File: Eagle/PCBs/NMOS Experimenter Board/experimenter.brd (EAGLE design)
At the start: 77.5 x 99.1 mm, 1441 parts, among them Q10 2N7002, Q11 2N7002, Q12 2N7002, Q13 2N7002, Q14 2N7002, Q15 2N7002, Q16 2N7002, Q17 2N7002, Q18 2N7002, Q19 2N7002, Q2 2N7002, Q20 2N7002, Q21 2N7002, Q22 2N7002, Q23 2N7002, Q24 2N7002, Q25 2N7002, Q26 2N7002, Q27 2N7002, Q28 2N7002, Q29 2N7002, Q3 2N7002, Q30 2N7002, Q31 2N7002, Q32 2N7002, Q33 2N7002, Q34 2N7002, Q35 2N7002, Q36 2N7002, Q37 2N7002, Q38 2N7002, Q39 2N7002, Q4 2N7002, Q40 2N7002, Q41 2N7002, Q42 2N7002, Q43 2N7002, Q44 2N7002, Q45 2N7002, Q46 2N7002, Q47 2N7002, Q48 2N7002, Q49 2N7002, Q5 2N7002, Q50 2N7002, Q51 2N7002, Q52 2N7002, Q53 2N7002, Q54 2N7002, Q55 2N7002, Q56 2N7002, Q57 2N7002, Q58 2N7002, Q59 2N7002, Q6 2N7002, Q60 2N7002, Q61 2N7002, Q62 2N7002, Q63 2N7002, Q64 2N7002, Q65 2N7002, Q66 2N7002, Q67 2N7002, Q68 2N7002, Q69 2N7002, Q7 2N7002, Q70 2N7002, Q71 2N7002, Q72 2N7002, Q73 2N7002, Q8 2N7002, Q9 2N7002, U1 74HC14PW, U2 74HC14PW

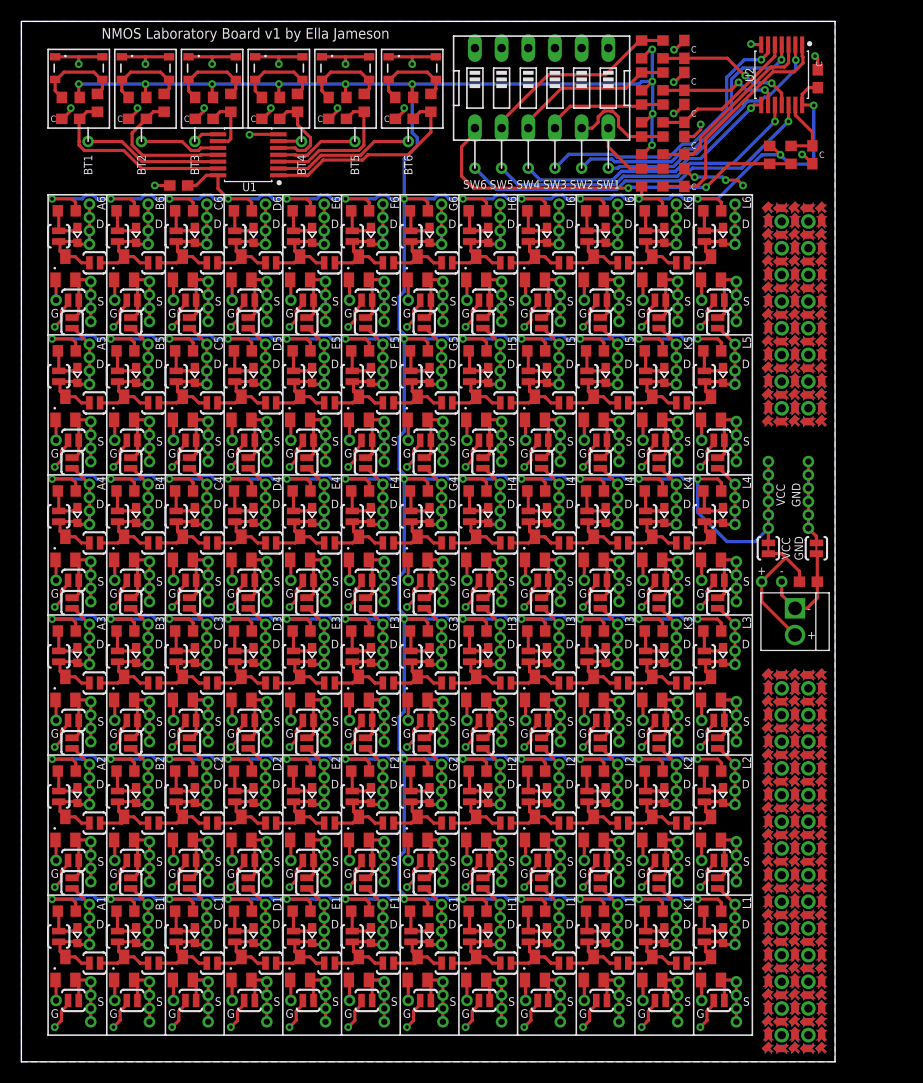
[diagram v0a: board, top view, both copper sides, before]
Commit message: Start rework on experimenter
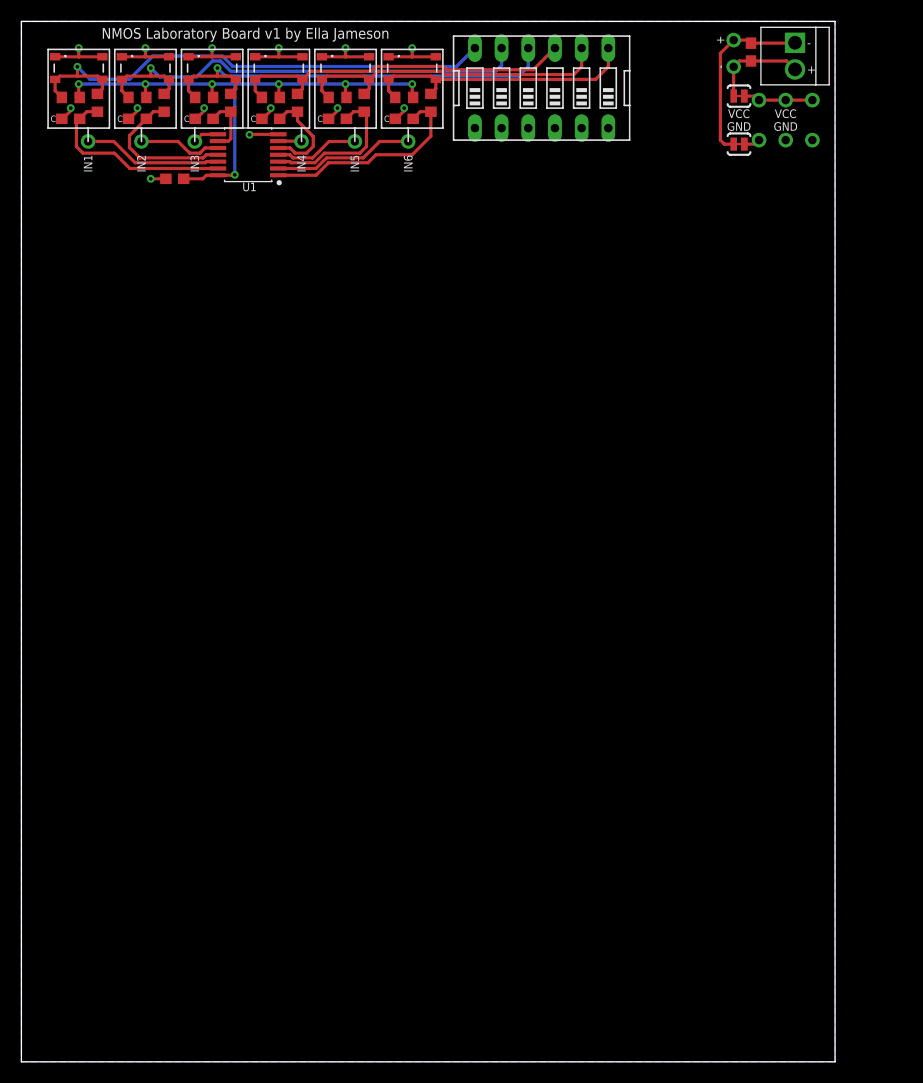
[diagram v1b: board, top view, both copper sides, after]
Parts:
- removed C10, C12, C13, C14, C15, C6, C8: 0.1u, ellajameson-core:C0603
- removed D10, D11, D12, D13, D14, D15, D16, D17, D18, D19, D2, D20, D21, D22, D23, D24, D25, D26, D27, D28, D29, D3, D30, D31, D32, D33, D34, D35, D36, D37, D38, D39, D4, D40, D41, D42, D43, D44, D45, D46, D47, D48, D49, D5, D50, D51, D52, D53, D54, D55, D56, D57, D58, D59, D6, D60, D61, D62, D63, D64, D65, D66, D67, D68, D69, D7, D70, D71, D72, D73, D8, D9: (no value), ellajameson-core:CHIP-LED0603
- removed DRAINA10, DRAINA11, DRAINA12, DRAINA13, DRAINA14, DRAINA15, DRAINA16, DRAINA17, DRAINA18, DRAINA19, DRAINA2, DRAINA20, DRAINA21, DRAINA22, DRAINA23, DRAINA24, DRAINA25, DRAINA26, DRAINA27, DRAINA28, DRAINA29, DRAINA3, DRAINA30, DRAINA31, DRAINA32, DRAINA33, DRAINA34, DRAINA35, DRAINA36, DRAINA37, DRAINA38, DRAINA39, DRAINA4, DRAINA40, DRAINA41, DRAINA42, DRAINA43, DRAINA44, DRAINA45, DRAINA46, DRAINA47, DRAINA48, DRAINA49, DRAINA5, DRAINA50, DRAINA51, DRAINA52, DRAINA53, DRAINA54, DRAINA55, DRAINA56, DRAINA57, DRAINA58, DRAINA59, DRAINA6, DRAINA60, DRAINA61, DRAINA62, DRAINA63, DRAINA64, DRAINA65, DRAINA66, DRAINA67, DRAINA68, DRAINA69, DRAINA7, DRAINA70, DRAINA71, DRAINA72, DRAINA73, DRAINA8, DRAINA9, DRAINB10, DRAINB11, DRAINB12, DRAINB13, DRAINB14, DRAINB15, DRAINB16, DRAINB17, DRAINB18, DRAINB19, DRAINB2, DRAINB20, DRAINB21, DRAINB22, DRAINB23, DRAINB24, DRAINB25, DRAINB26, DRAINB27, DRAINB28, DRAINB29, DRAINB3, DRAINB30, DRAINB31, DRAINB32, DRAINB33, DRAINB34, DRAINB35, DRAINB36, DRAINB37, DRAINB38, DRAINB39, DRAINB4, DRAINB40, DRAINB41, DRAINB42, DRAINB43, DRAINB44, DRAINB45, DRAINB46, DRAINB47, DRAINB48, DRAINB49, DRAINB5, DRAINB50, DRAINB51, DRAINB52, DRAINB53, DRAINB54, DRAINB55, DRAINB56, DRAINB57, DRAINB58, DRAINB59, DRAINB6, DRAINB60, DRAINB61, DRAINB62, DRAINB63, DRAINB64, DRAINB65, DRAINB66, DRAINB67, DRAINB68, DRAINB69, DRAINB7, DRAINB70, DRAINB71, DRAINB72, DRAINB73, DRAINB8, DRAINB9, DRAINC10, DRAINC11, DRAINC12, DRAINC13, DRAINC14, DRAINC15, DRAINC16, DRAINC17, DRAINC18, DRAINC19, DRAINC2, DRAINC20, DRAINC21, DRAINC22, DRAINC23, DRAINC24, DRAINC25, DRAINC26, DRAINC27, DRAINC28, DRAINC29, DRAINC3, DRAINC30, DRAINC31, DRAINC32, DRAINC33, DRAINC34, DRAINC35, DRAINC36, DRAINC37, DRAINC38, DRAINC39, DRAINC4, DRAINC40, DRAINC41, DRAINC42, DRAINC43, DRAINC44, DRAINC45, DRAINC46, DRAINC47, DRAINC48, DRAINC49, DRAINC5, DRAINC50, DRAINC51, DRAINC52, DRAINC53, DRAINC54, DRAINC55, DRAINC56, DRAINC57, DRAINC58, DRAINC59, DRAINC6, DRAINC60, DRAINC61, DRAINC62, DRAINC63, DRAINC64, DRAINC65, DRAINC66, DRAINC67, DRAINC68, DRAINC69, DRAINC7, DRAINC70, DRAINC71, DRAINC72, DRAINC73, DRAINC8, DRAINC9, DRAIND10, DRAIND11, DRAIND12, DRAIND13, DRAIND14, DRAIND15, DRAIND16, DRAIND17, DRAIND18, DRAIND19, DRAIND2, DRAIND20, DRAIND21, DRAIND22, DRAIND23, DRAIND24, DRAIND25, DRAIND26, DRAIND27, DRAIND28, DRAIND29, DRAIND3, DRAIND30, DRAIND31, DRAIND32, DRAIND33, DRAIND34, DRAIND35, DRAIND36, DRAIND37, DRAIND38, DRAIND39, DRAIND4, DRAIND40, DRAIND41, DRAIND42, DRAIND43, DRAIND44, DRAIND45, DRAIND46, DRAIND47, DRAIND48, DRAIND49, DRAIND5, DRAIND50, DRAIND51, DRAIND52, DRAIND53, DRAIND54, DRAIND55, DRAIND56, DRAIND57, DRAIND58, DRAIND59, DRAIND6, DRAIND60, DRAIND61, DRAIND62, DRAIND63, DRAIND64, DRAIND65, DRAIND66, DRAIND67, DRAIND68, DRAIND69, DRAIND7, DRAIND70, DRAIND71, DRAIND72, DRAIND73, DRAIND8, DRAIND9, GATE10, GATE11, GATE12, GATE13, GATE14, GATE15, GATE16, GATE17, GATE18, GATE19, GATE2, GATE20, GATE21, GATE22, GATE23, GATE24, GATE25, GATE26, GATE27, GATE28, GATE29, GATE3, GATE30, GATE31, GATE32, GATE33, GATE34, GATE35, GATE36, GATE37, GATE38, GATE39, GATE4, GATE40, GATE41, GATE42, GATE43, GATE44, GATE45, GATE46, GATE47, GATE48, GATE49, GATE5, GATE50, GATE51, GATE52, GATE53, GATE54, GATE55, GATE56, GATE57, GATE58, GATE59, GATE6, GATE60, GATE61, GATE62, GATE63, GATE64, GATE65, GATE66, GATE67, GATE68, GATE69, GATE7, GATE70, GATE71, GATE72, GATE73, GATE8, GATE9, SO1, SO2, SO3, SO4, SO5, SO6, SOURCEA10, SOURCEA11, SOURCEA12, SOURCEA13, SOURCEA14, SOURCEA15, SOURCEA16, SOURCEA17, SOURCEA18, SOURCEA19, SOURCEA2, SOURCEA20, SOURCEA21, SOURCEA22, SOURCEA23, SOURCEA24, SOURCEA25, SOURCEA26, SOURCEA27, SOURCEA28, SOURCEA29, SOURCEA3, SOURCEA30, SOURCEA31, SOURCEA32, SOURCEA33, SOURCEA34, SOURCEA35, SOURCEA36, SOURCEA37, SOURCEA38, SOURCEA39, SOURCEA4, SOURCEA40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: TPWIRE, ellajameson-core:TP_TH_WIRE
- removed JD10, JD11, JD12, JD13, JD14, JD17, JD18, JD19, JD2, JD20, JD21, JD22, JD23, JD24, JD25, JD26, JD27, JD28, JD29, JD3, JD30, JD31, JD32, JD33, JD34, JD35, JD36, JD37, JD38, JD39, JD4, JD40, JD41, JD42, JD43, JD44, JD45, JD46, JD47, JD48, JD49, JD5, JD50, JD51, JD52, JD53, JD54, JD55, JD56, JD57, JD58, JD59, JD6, JD60, JD61, JD62, JD63, JD64, JD65, JD66, JD68, JD7, JD70, JD72, JD8, JD9, JN10, JN11, JN12, JN13, JN14, JN15, JN16, JN17, JN18, JN19, JN2, JN20, JN21, JN22, JN23, JN24, JN25, JN26, JN27, JN28, JN29, JN3, JN30, JN31, JN32, JN33, JN34, JN35, JN36, JN37, JN38, JN39, JN4, JN40, JN41, JN42, JN43, JN44, JN45, JN46, JN47, JN48, JN49, JN5, JN50, JN51, JN52, JN53, JN54, JN55, JN56, JN57, JN58, JN59, JN6, JN60, JN61, JN62, JN63, JN64, JN65, JN66, JN67, JN68, JN69, JN7, JN70, JN71, JN72, JN73, JN8, JN9, JP10, JP11, JP12, JP13, JP14, JP15, JP16, JP17, JP18, JP19, JP2, JP20, JP21, JP22, JP23, JP24, JP25, JP26, JP27, JP28, JP29, JP3, JP30, JP31, JP32, JP33, JP34, JP35, JP36, JP37, JP38, JP39, JP4, JP40, JP41, JP42, JP43, JP44, JP45, JP46, JP47, JP48, JP49, JP5, JP50, JP51, JP52, JP53, JP54, JP55, JP56, JP57, JP58, JP59, JP6, JP60, JP61, JP62, JP63, JP64, JP65, JP66, JP67, JP68, JP69, JP7, JP70, JP71, JP72, JP73, JP8, JP9, JS10, JS11, JS12, JS13, JS16, JS17, JS26, JS27, JS28, JS29, JS30, JS31, JS32, JS33, JS34, JS35, JS36, JS37, JS38, JS39, JS4, JS40, JS41, JS42, JS43, JS44, JS45, JS46, JS47, JS48, JS49, JS5, JS50, JS51, JS52, JS53, JS54, JS55, JS56, JS57, JS58, JS59, JS6, JS60, JS61, JS62, JS63, JS64, JS65, JS66, JS67, JS68, JS69, JS7, JS70, JS71, JS72, JS73, JS8, JS9: SJ_NO, ellajameson-core:SJ_2S-NO
- removed Q10, Q11, Q12, Q13, Q14, Q15, Q16, Q17, Q18, Q19, Q2, Q20, Q21, Q22, Q23, Q24, Q25, Q26, Q27, Q28, Q29, Q3, Q30, Q31, Q32, Q33, Q34, Q35, Q36, Q37, Q38, Q39, Q4, Q40, Q41, Q42, Q43, Q44, Q45, Q46, Q47, Q48, Q49, Q5, Q50, Q51, Q52, Q53, Q54, Q55, Q56, Q57, Q58, Q59, Q6, Q60, Q61, Q62, Q63, Q64, Q65, Q66, Q67, Q68, Q69, Q7, Q70, Q71, Q72, Q73, Q8, Q9: 2N7002, ellajameson-core:SOT23
- removed R1, R74, R79, R80, R83, R84, R87, R88, R91, R92, R95, R96: 10k, ellajameson-core:R0603
- removed R10, R11, R12, R13, R14, R15, R16, R17, R18, R19, R2, R20, R21, R22, R23, R24, R25, R26, R27, R28, R29, R3, R30, R31, R32, R33, R34, R35, R36, R37, R38, R39, R4, R40, R41, R42, R43, R44, R45, R46, R47, R48, R49, R5, R50, R51, R52, R53, R54, R55, R56, R57, R58, R59, R6, R60, R61, R62, R63, R64, R65, R66, R67, R68, R69, R7, R70, R71, R72, R73, R8, R9: (no value), ellajameson-core:R0603
- removed U$1, U$101, U$105, U$109, U$113, U$117, U$121, U$125, U$162, U$166, U$170, U$174, U$182, U$186, U$190, U$194, U$198, U$202, U$206, U$21, U$210, U$214, U$218, U$222, U$226, U$25, U$29, U$33, U$37, U$41, U$45, U$49, U$53, U$57, U$61, U$65, U$69, U$73, U$77, U$81, U$85, U$89, U$93, U$97: PROTOPADTHT, ellajameson-core:PROTOPAD-THT
- removed U$10, U$100, U$104, U$108, U$112, U$116, U$12, U$120, U$124, U$128, U$130, U$132, U$134, U$136, U$138, U$14, U$140, U$142, U$144, U$145, U$147, U$149, U$151, U$153, U$154, U$156, U$158, U$16, U$160, U$165, U$169, U$173, U$177, U$178, U$18, U$180, U$185, U$189, U$193, U$197, U$20, U$201, U$205, U$209, U$213, U$217, U$221, U$225, U$229, U$230, U$24, U$28, U$32, U$36, U$4, U$40, U$44, U$48, U$52, U$56, U$6, U$60, U$64, U$68, U$72, U$76, U$8, U$80, U$84, U$88, U$92, U$96: (no value), ellajameson-core:PROTOPAD-CENTER
- removed U$102, U$103, U$106, U$107, U$11, U$110, U$111, U$114, U$115, U$118, U$119, U$122, U$123, U$126, U$127, U$129, U$13, U$131, U$133, U$135, U$137, U$139, U$141, U$143, U$146, U$148, U$15, U$150, U$152, U$155, U$157, U$159, U$161, U$163, U$164, U$167, U$168, U$17, U$171, U$172, U$175, U$176, U$179, U$181, U$183, U$184, U$187, U$188, U$19, U$191, U$192, U$195, U$196, U$199, U$2, U$200, U$203, U$204, U$207, U$208, U$211, U$212, U$215, U$216, U$219, U$22, U$220, U$223, U$224, U$227, U$228, U$23, U$26, U$27, U$3, U$30, U$31, U$34, U$35, U$38, U$39, U$42, U$43, U$46, U$47, U$5, U$50, U$51, U$54, U$55, U$58, U$59, U$62, U$63, U$66, U$67, U$7, U$70, U$71, U$74, U$75, U$78, U$79, U$82, U$83, U$86, U$87, U$9, U$90, U$91, U$94, U$95, U$98, U$99: (no value), ellajameson-core:PROTOPAD-BETWEEN
- removed U2: 74HC14PW, ellajameson-core:TSSOP14
- B1, B2, B3, B4, B5, B6, VCC1, VCC2, VCC3, VIN+1, VIN-1, VSS1, VSS2, VSS3: value TPWIRE -> TPTHT; device ellajameson-core:TP_TH_WIRE -> ellajameson-core:PROTOPAD-THT
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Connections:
- removed net N$1: D2.A, JP2.2, R2.1
- removed net N$10: D3.C, DRAINA3.TP, DRAINB3.TP, DRAINC3.TP, DRAIND3.TP, JD2.1, JD3.2, JP3.1, JS5.1, Q3.3
- removed net N$100: GATE25.TP, Q25.1
- removed net N$101: D26.A, JP26.2, R26.1
- removed net N$102: D26.C, DRAINA26.TP, DRAINB26.TP, DRAINC26.TP, DRAIND26.TP, JD26.2, JP26.1, JS34.1, Q26.3
- removed net N$103: JN26.2, JS26.2, Q26.2, SOURCEA26.TP, SOURCEB26.TP, SOURCEC26.TP, SOURCED26.TP
- removed net N$104: GATE26.TP, Q26.1
- removed net N$105: D27.A, JP27.2, R27.1
- removed net N$106: D27.C, DRAINA27.TP, DRAINB27.TP, DRAINC27.TP, DRAIND27.TP, JD26.1, JD27.2, JP27.1, JS35.1, Q27.3
- removed net N$107: JN27.2, JS27.2, Q27.2, SOURCEA27.TP, SOURCEB27.TP, SOURCEC27.TP, SOURCED27.TP
- removed net N$108: GATE27.TP, Q27.1
- removed net N$109: D28.A, JP28.2, R28.1
- removed net N$11: JN3.2, Q3.2, SOURCEA3.TP, SOURCEB3.TP, SOURCEC3.TP, SOURCED3.TP
- removed net N$110: D28.C, DRAINA28.TP, DRAINB28.TP, DRAINC28.TP, DRAIND28.TP, JD27.1, JD28.2, JP28.1, JS36.1, Q28.3
- removed net N$111: JN28.2, JS28.2, Q28.2, SOURCEA28.TP, SOURCEB28.TP, SOURCEC28.TP, SOURCED28.TP
- removed net N$112: GATE28.TP, Q28.1
- removed net N$113: D29.A, JP29.2, R29.1
- removed net N$114: D29.C, DRAINA29.TP, DRAINB29.TP, DRAINC29.TP, DRAIND29.TP, JD28.1, JD29.2, JP29.1, JS37.1, Q29.3
- removed net N$115: JN29.2, JS29.2, Q29.2, SOURCEA29.TP, SOURCEB29.TP, SOURCEC29.TP, SOURCED29.TP
- removed net N$116: GATE29.TP, Q29.1
- removed net N$117: D30.A, JP30.2, R30.1
- removed net N$118: D30.C, DRAINA30.TP, DRAINB30.TP, DRAINC30.TP, DRAIND30.TP, JD29.1, JD30.2, JP30.1, JS38.1, Q30.3
- removed net N$119: JN30.2, JS30.2, Q30.2, SOURCEA30.TP, SOURCEB30.TP, SOURCEC30.TP, SOURCED30.TP
- removed net N$12: GATE3.TP, Q3.1
- removed net N$120: GATE30.TP, Q30.1
- removed net N$121: D31.A, JP31.2, R31.1
- removed net N$122: D31.C, DRAINA31.TP, DRAINB31.TP, DRAINC31.TP, DRAIND31.TP, JD30.1, JD31.2, JP31.1, JS39.1, Q31.3
- removed net N$123: JN31.2, JS31.2, Q31.2, SOURCEA31.TP, SOURCEB31.TP, SOURCEC31.TP, SOURCED31.TP
- removed net N$124: GATE31.TP, Q31.1
- removed net N$125: D32.A, JP32.2, R32.1
- removed net N$126: D32.C, DRAINA32.TP, DRAINB32.TP, DRAINC32.TP, DRAIND32.TP, JD31.1, JD32.2, JP32.1, JS40.1, Q32.3
- removed net N$127: JN32.2, JS32.2, Q32.2, SOURCEA32.TP, SOURCEB32.TP, SOURCEC32.TP, SOURCED32.TP
- removed net N$128: GATE32.TP, Q32.1
- removed net N$129: D33.A, JP33.2, R33.1
- removed net N$13: D4.A, JP4.2, R4.1
- removed net N$130: D33.C, DRAINA33.TP, DRAINB33.TP, DRAINC33.TP, DRAIND33.TP, JD32.1, JD33.2, JP33.1, JS41.1, Q33.3
- removed net N$131: JN33.2, JS33.2, Q33.2, SOURCEA33.TP, SOURCEB33.TP, SOURCEC33.TP, SOURCED33.TP
- removed net N$132: GATE33.TP, Q33.1
- removed net N$133: D34.A, JP34.2, R34.1
- removed net N$134: D34.C, DRAINA34.TP, DRAINB34.TP, DRAINC34.TP, DRAIND34.TP, JD34.2, JP34.1, JS42.1, Q34.3
- removed net N$135: JN34.2, JS34.2, Q34.2, SOURCEA34.TP, SOURCEB34.TP, SOURCEC34.TP, SOURCED34.TP
- removed net N$136: GATE34.TP, Q34.1
- removed net N$137: D35.A, JP35.2, R35.1
- removed net N$138: D35.C, DRAINA35.TP, DRAINB35.TP, DRAINC35.TP, DRAIND35.TP, JD34.1, JD35.2, JP35.1, JS43.1, Q35.3
- removed net N$139: JN35.2, JS35.2, Q35.2, SOURCEA35.TP, SOURCEB35.TP, SOURCEC35.TP, SOURCED35.TP
- removed net N$14: D4.C, DRAINA4.TP, DRAINB4.TP, DRAINC4.TP, DRAIND4.TP, JD33.1, JD4.2, JP4.1, JS6.1, Q4.3
- removed net N$140: GATE35.TP, Q35.1
- removed net N$141: D36.A, JP36.2, R36.1
- removed net N$142: D36.C, DRAINA36.TP, DRAINB36.TP, DRAINC36.TP, DRAIND36.TP, JD35.1, JD36.2, JP36.1, JS44.1, Q36.3
- removed net N$143: JN36.2, JS36.2, Q36.2, SOURCEA36.TP, SOURCEB36.TP, SOURCEC36.TP, SOURCED36.TP
- removed net N$144: GATE36.TP, Q36.1
- removed net N$145: D37.A, JP37.2, R37.1
- removed net N$146: D37.C, DRAINA37.TP, DRAINB37.TP, DRAINC37.TP, DRAIND37.TP, JD36.1, JD37.2, JP37.1, JS45.1, Q37.3
- removed net N$147: JN37.2, JS37.2, Q37.2, SOURCEA37.TP, SOURCEB37.TP, SOURCEC37.TP, SOURCED37.TP
- removed net N$148: GATE37.TP, Q37.1
- removed net N$149: D38.A, JP38.2, R38.1
- removed net N$15: JN4.2, JS4.2, Q4.2, SOURCEA4.TP, SOURCEB4.TP, SOURCEC4.TP, SOURCED4.TP
- removed net N$150: D38.C, DRAINA38.TP, DRAINB38.TP, DRAINC38.TP, DRAIND38.TP, JD37.1, JD38.2, JP38.1, JS46.1, Q38.3
- removed net N$151: JN38.2, JS38.2, Q38.2, SOURCEA38.TP, SOURCEB38.TP, SOURCEC38.TP, SOURCED38.TP
- removed net N$152: GATE38.TP, Q38.1
- removed net N$153: D39.A, JP39.2, R39.1
- removed net N$154: D39.C, DRAINA39.TP, DRAINB39.TP, DRAINC39.TP, DRAIND39.TP, JD38.1, JD39.2, JP39.1, JS47.1, Q39.3
- removed net N$155: JN39.2, JS39.2, Q39.2, SOURCEA39.TP, SOURCEB39.TP, SOURCEC39.TP, SOURCED39.TP
- removed net N$156: GATE39.TP, Q39.1
- removed net N$157: D40.A, JP40.2, R40.1
- removed net N$158: D40.C, DRAINA40.TP, DRAINB40.TP, DRAINC40.TP, DRAIND40.TP, JD39.1, JD40.2, JP40.1, JS48.1, Q40.3
- removed net N$159: JN40.2, JS40.2, Q40.2, SOURCEA40.TP, SOURCEB40.TP, SOURCEC40.TP, SOURCED40.TP
- removed net N$16: GATE4.TP, Q4.1
- removed net N$160: GATE40.TP, Q40.1
- removed net N$161: D41.A, JP41.2, R41.1
- removed net N$162: D41.C, DRAINA41.TP, DRAINB41.TP, DRAINC41.TP, DRAIND41.TP, JD40.1, JD41.2, JP41.1, JS49.1, Q41.3
- removed net N$163: JN41.2, JS41.2, Q41.2, SOURCEA41.TP, SOURCEB41.TP, SOURCEC41.TP, SOURCED41.TP
- removed net N$164: GATE41.TP, Q41.1
- removed net N$165: D42.A, JP42.2, R42.1
- removed net N$166: D42.C, DRAINA42.TP, DRAINB42.TP, DRAINC42.TP, DRAIND42.TP, JD42.2, JP42.1, JS50.1, Q42.3
- removed net N$167: JN42.2, JS42.2, Q42.2, SOURCEA42.TP, SOURCEB42.TP, SOURCEC42.TP, SOURCED42.TP
- removed net N$168: GATE42.TP, Q42.1
- removed net N$169: D43.A, JP43.2, R43.1
- removed net N$17: D5.A, JP5.2, R5.1
- removed net N$170: D43.C, DRAINA43.TP, DRAINB43.TP, DRAINC43.TP, DRAIND43.TP, JD42.1, JD43.2, JP43.1, JS51.1, Q43.3
- removed net N$171: JN43.2, JS43.2, Q43.2, SOURCEA43.TP, SOURCEB43.TP, SOURCEC43.TP, SOURCED43.TP
- removed net N$172: GATE43.TP, Q43.1
- removed net N$173: D44.A, JP44.2, R44.1
- removed net N$174: D44.C, DRAINA44.TP, DRAINB44.TP, DRAINC44.TP, DRAIND44.TP, JD43.1, JD44.2, JP44.1, JS52.1, Q44.3
- removed net N$175: JN44.2, JS44.2, Q44.2, SOURCEA44.TP, SOURCEB44.TP, SOURCEC44.TP, SOURCED44.TP
- removed net N$176: GATE44.TP, Q44.1
- removed net N$177: D45.A, JP45.2, R45.1
- removed net N$178: D45.C, DRAINA45.TP, DRAINB45.TP, DRAINC45.TP, DRAIND45.TP, JD44.1, JD45.2, JP45.1, JS53.1, Q45.3
- removed net N$179: JN45.2, JS45.2, Q45.2, SOURCEA45.TP, SOURCEB45.TP, SOURCEC45.TP, SOURCED45.TP
- removed net N$18: D5.C, DRAINA5.TP, DRAINB5.TP, DRAINC5.TP, DRAIND5.TP, JD4.1, JD5.2, JP5.1, JS7.1, Q5.3
- removed net N$180: GATE45.TP, Q45.1
- removed net N$181: D46.A, JP46.2, R46.1
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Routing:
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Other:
- board text added: "IN1"
- board text added: "IN2"
- board text added: "IN3"
- board text added: "IN4"
- board text added: "IN5"
- board text added: "IN6"
- board text removed: "A1"
- board text removed: "A2"
- board text removed: "A3"
- board text removed: "A4"
- board text removed: "A5"
- board text removed: "A6"
- board text removed: "B1"
- board text removed: "B2"
- board text removed: "B3"
- board text removed: "B4"
- board text removed: "B5"
- board text removed: "B6"
- board text removed: "BT1"
- board text removed: "BT2"
- board text removed: "BT3"
- board text removed: "BT4"
- board text removed: "BT5"
- board text removed: "BT6"
- board text removed: "C1"
- board text removed: "C2"
- board text removed: "C3"
- board text removed: "C4"
- board text removed: "C5"
- board text removed: "C6"
- board text removed: "D"
- board text removed: "D1"
- board text removed: "D2"
- board text removed: "D3"
- board text removed: "D4"
- board text removed: "D5"
- board text removed: "D6"
- board text removed: "E1"
- board text removed: "E2"
- board text removed: "E3"
- board text removed: "E4"
- board text removed: "E5"
- board text removed: "E6"
- board text removed: "F1"
- board text removed: "F2"
- board text removed: "F3"
- board text removed: "F4"
- board text removed: "F5"
- board text removed: "F6"
- board text removed: "G"
- board text removed: "G1"
- board text removed: "G2"
- board text removed: "G3"
- board text removed: "G4"
- board text removed: "G5"
- board text removed: "G6"
- board text removed: "H1"
- board text removed: "H2"
- board text removed: "H3"
- board text removed: "H4"
- board text removed: "H5"
- board text removed: "H6"
- board text removed: "I1"
- board text removed: "I2"
- board text removed: "I3"
- board text removed: "I4"
- board text removed: "I5"
- board text removed: "I6"
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
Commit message: Wow, 92 transistors and 8 LEDs
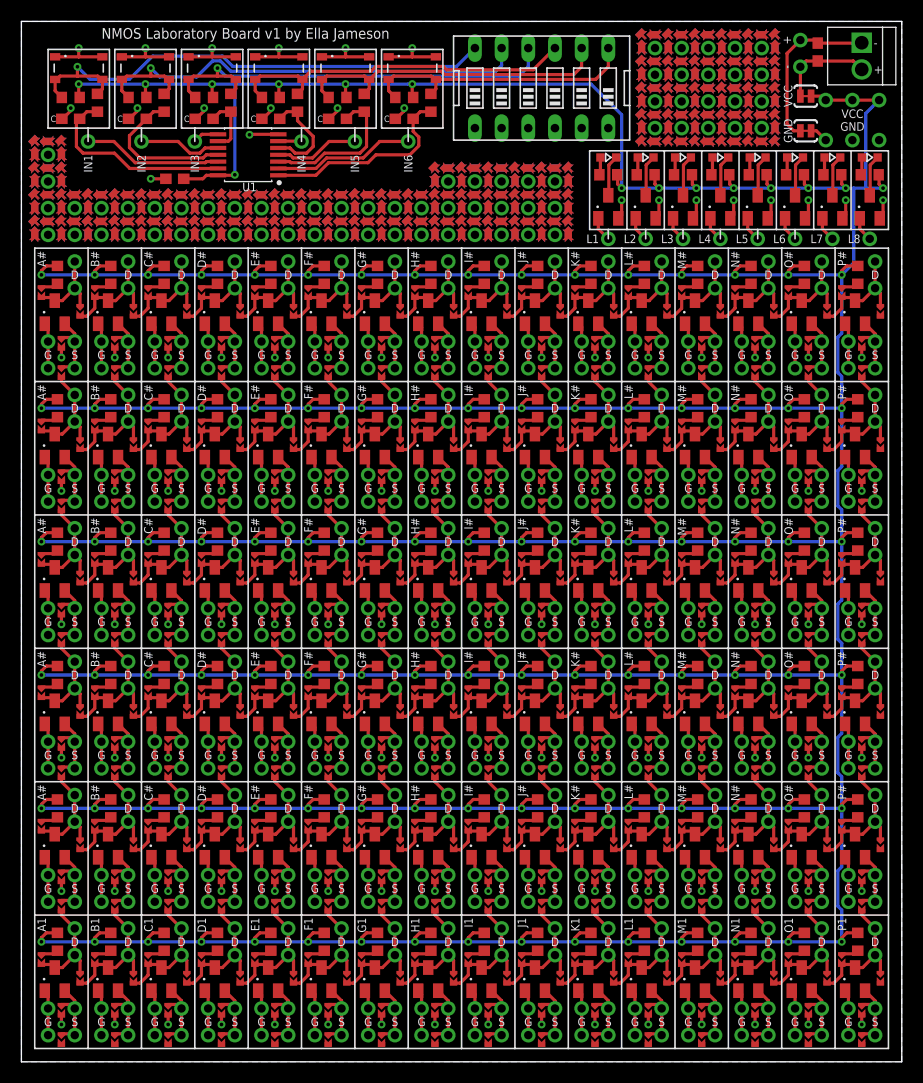
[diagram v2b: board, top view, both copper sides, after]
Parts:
- added D2, D3, D4, D5, D6, D7, D8, D9: (no value), ellajameson-core:CHIP-LED0603
- added DRAINA100, DRAINA101, DRAINA102, DRAINA103, DRAINA104, DRAINA105, DRAINA106, DRAINA107, DRAINA108, DRAINA109, DRAINA110, DRAINA111, DRAINA112, DRAINA2, DRAINA21, DRAINA22, DRAINA23, DRAINA24, DRAINA25, DRAINA26, DRAINA27, DRAINA28, DRAINA29, DRAINA3, DRAINA30, DRAINA31, DRAINA32, DRAINA33, DRAINA34, DRAINA35, DRAINA36, DRAINA37, DRAINA38, DRAINA39, DRAINA4, DRAINA40, DRAINA41, DRAINA42, DRAINA43, DRAINA44, DRAINA45, DRAINA46, DRAINA47, DRAINA48, DRAINA49, DRAINA5, DRAINA50, DRAINA51, DRAINA52, DRAINA53, DRAINA54, DRAINA55, DRAINA56, DRAINA57, DRAINA58, DRAINA59, DRAINA60, DRAINA61, DRAINA62, DRAINA63, DRAINA64, DRAINA65, DRAINA66, DRAINA67, DRAINA68, DRAINA69, DRAINA70, DRAINA71, DRAINA72, DRAINA73, DRAINA74, DRAINA75, DRAINA76, DRAINA77, DRAINA78, DRAINA79, DRAINA80, DRAINA81, DRAINA82, DRAINA83, DRAINA84, DRAINA85, DRAINA86, DRAINA87, DRAINA88, DRAINA89, DRAINA90, DRAINA91, DRAINA92, DRAINA93, DRAINA94, DRAINA95, DRAINA96, DRAINA97, DRAINA98, DRAINA99, DRAINB100, DRAINB101, DRAINB102, DRAINB103, DRAINB104, DRAINB105, DRAINB106, DRAINB107, DRAINB108, DRAINB109, DRAINB110, DRAINB111, DRAINB112, DRAINB2, DRAINB21, DRAINB22, DRAINB23, DRAINB24, DRAINB25, DRAINB26, DRAINB27, DRAINB28, DRAINB29, DRAINB3, DRAINB30, DRAINB31, DRAINB32, DRAINB33, DRAINB34, DRAINB35, DRAINB36, DRAINB37, DRAINB38, DRAINB39, DRAINB4, DRAINB40, DRAINB41, DRAINB42, DRAINB43, DRAINB44, DRAINB45, DRAINB46, DRAINB47, DRAINB48, DRAINB49, DRAINB5, DRAINB50, DRAINB51, DRAINB52, DRAINB53, DRAINB54, DRAINB55, DRAINB56, DRAINB57, DRAINB58, DRAINB59, DRAINB60, DRAINB61, DRAINB62, DRAINB63, DRAINB64, DRAINB65, DRAINB66, DRAINB67, DRAINB68, DRAINB69, DRAINB70, DRAINB71, DRAINB72, DRAINB73, DRAINB74, DRAINB75, DRAINB76, DRAINB77, DRAINB78, DRAINB79, DRAINB80, DRAINB81, DRAINB82, DRAINB83, DRAINB84, DRAINB85, DRAINB86, DRAINB87, DRAINB88, DRAINB89, DRAINB90, DRAINB91, DRAINB92, DRAINB93, DRAINB94, DRAINB95, DRAINB96, DRAINB97, DRAINB98, DRAINB99, GATEA100, GATEA101, GATEA102, GATEA103, GATEA104, GATEA105, GATEA106, GATEA107, GATEA108, GATEA109, GATEA110, GATEA111, GATEA112, GATEA2, GATEA21, GATEA22, GATEA23, GATEA24, GATEA25, GATEA26, GATEA27, GATEA28, GATEA29, GATEA3, GATEA30, GATEA31, GATEA32, GATEA33, GATEA34, GATEA35, GATEA36, GATEA37, GATEA38, GATEA39, GATEA4, GATEA40, GATEA41, GATEA42, GATEA43, GATEA44, GATEA45, GATEA46, GATEA47, GATEA48, GATEA49, GATEA5, GATEA50, GATEA51, GATEA52, GATEA53, GATEA54, GATEA55, GATEA56, GATEA57, GATEA58, GATEA59, GATEA60, GATEA61, GATEA62, GATEA63, GATEA64, GATEA65, GATEA66, GATEA67, GATEA68, GATEA69, GATEA70, GATEA71, GATEA72, GATEA73, GATEA74, GATEA75, GATEA76, GATEA77, GATEA78, GATEA79, GATEA80, GATEA81, GATEA82, GATEA83, GATEA84, GATEA85, GATEA86, GATEA87, GATEA88, GATEA89, GATEA90, GATEA91, GATEA92, GATEA93, GATEA94, GATEA95, GATEA96, GATEA97, GATEA98, GATEA99, GATEB100, GATEB101, GATEB102, GATEB103, GATEB104, GATEB105, GATEB106, GATEB107, GATEB108, GATEB109, GATEB110, GATEB111, GATEB112, GATEB2, GATEB21, GATEB22, GATEB23, GATEB24, GATEB25, GATEB26, GATEB27, GATEB28, GATEB29, GATEB3, GATEB30, GATEB31, GATEB32, GATEB33, GATEB34, GATEB35, GATEB36, GATEB37, GATEB38, GATEB39, GATEB4, GATEB40, GATEB41, GATEB42, GATEB43, GATEB44, GATEB45, GATEB46, GATEB47, GATEB48, GATEB49, GATEB5, GATEB50, GATEB51, GATEB52, GATEB53, GATEB54, GATEB55, GATEB56, GATEB57, GATEB58, GATEB59, GATEB60, GATEB61, GATEB62, GATEB63, GATEB64, GATEB65, GATEB66, GATEB67, GATEB68, GATEB69, GATEB70, GATEB71, GATEB72, GATEB73, GATEB74, GATEB75, GATEB76, GATEB77, GATEB78, GATEB79, GATEB80, GATEB81, GATEB82, GATEB83, GATEB84, GATEB85, GATEB86, GATEB87, GATEB88, GATEB89, GATEB90, GATEB91, GATEB92, GATEB93, GATEB94, GATEB95, GATEB96, GATEB97, GATEB98, GATEB99, LED2, LED3, LED4, LED5, LED6, LED7, LED8, LED9, SOURCEA100, SOURCEA101, SOURCEA102, SOURCEA103, SOURCEA104, SOURCEA105, SOURCEA106, SOURCEA107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: TPTHT, ellajameson-core:PROTOPAD-THT-PAD
- added JD100, JD101, JD102, JD103, JD104, JD105, JD106, JD107, JD108, JD109, JD110, JD111, JD112, JD2, JD21, JD22, JD23, JD24, JD25, JD26, JD27, JD28, JD29, JD3, JD30, JD31, JD32, JD33, JD34, JD35, JD36, JD37, JD38, JD39, JD4, JD40, JD41, JD42, JD43, JD44, JD45, JD46, JD47, JD48, JD49, JD5, JD50, JD51, JD52, JD53, JD54, JD55, JD56, JD57, JD58, JD59, JD60, JD61, JD62, JD63, JD64, JD65, JD66, JD67, JD68, JD69, JD70, JD71, JD72, JD73, JD74, JD75, JD76, JD77, JD78, JD79, JD80, JD81, JD82, JD83, JD84, JD85, JD86, JD87, JD88, JD89, JD90, JD91, JD92, JD93, JD94, JD95, JD96, JD97, JD98, JD99, JN100, JN101, JN102, JN103, JN104, JN105, JN106, JN107, JN108, JN109, JN110, JN111, JN112, JN2, JN21, JN22, JN23, JN24, JN25, JN26, JN27, JN28, JN29, JN3, JN30, JN31, JN32, JN33, JN34, JN35, JN36, JN37, JN38, JN39, JN4, JN40, JN41, JN42, JN43, JN44, JN45, JN46, JN47, JN48, JN49, JN5, JN50, JN51, JN52, JN53, JN54, JN55, JN56, JN57, JN58, JN59, JN60, JN61, JN62, JN63, JN64, JN65, JN66, JN67, JN68, JN69, JN70, JN71, JN72, JN73, JN74, JN75, JN76, JN77, JN78, JN79, JN80, JN81, JN82, JN83, JN84, JN85, JN86, JN87, JN88, JN89, JN90, JN91, JN92, JN93, JN94, JN95, JN96, JN97, JN98, JN99, JP100, JP101, JP102, JP103, JP104, JP105, JP106, JP107, JP108, JP109, JP110, JP111, JP112, JP2, JP21, JP22, JP23, JP24, JP25, JP26, JP27, JP28, JP29, JP3, JP30, JP31, JP32, JP33, JP34, JP35, JP36, JP37, JP38, JP39, JP4, JP40, JP41, JP42, JP43, JP44, JP45, JP46, JP47, JP48, JP49, JP5, JP50, JP51, JP52, JP53, JP54, JP55, JP56, JP57, JP58, JP59, JP60, JP61, JP62, JP63, JP64, JP65, JP66, JP67, JP68, JP69, JP70, JP71, JP72, JP73, JP74, JP75, JP76, JP77, JP78, JP79, JP80, JP81, JP82, JP83, JP84, JP85, JP86, JP87, JP88, JP89, JP90, JP91, JP92, JP93, JP94, JP95, JP96, JP97, JP98, JP99, JS100, JS101, JS102, JS103, JS104, JS105, JS106, JS107, JS108, JS109, JS110, JS111, JS112, JS2, JS21, JS22, JS23, JS24, JS25, JS26, JS27, JS28, JS29, JS3, JS30, JS31, JS32, JS33, JS34, JS35, JS36, JS37, JS38, JS39, JS4, JS40, JS41, JS42, JS43, JS44, JS45, JS46, JS47, JS48, JS49, JS5, JS50, JS51, JS52, JS53, JS54, JS55, JS56, JS57, JS58, JS59, JS60, JS61, JS62, JS63, JS64, JS65, JS66, JS67, JS68, JS69, JS70, JS71, JS72, JS73, JS74, JS75, JS76, JS77, JS78, JS79, JS80, JS81, JS82, JS83, JS84, JS85, JS86, JS87, JS88, JS89, JS90, JS91, JS92, JS93, JS94, JS95, JS96, JS97, JS98, JS99: SJ_NO_THIN, ellajameson-core:SJ_2S-NO-THIN
- added Q100, Q101, Q102, Q103, Q104, Q105, Q106, Q107, Q108, Q109, Q110, Q111, Q112, Q113, Q114, Q115, Q116, Q117, Q118, Q119, Q120, Q2, Q25, Q26, Q27, Q28, Q29, Q3, Q30, Q31, Q32, Q33, Q34, Q35, Q36, Q37, Q38, Q39, Q4, Q40, Q41, Q42, Q43, Q44, Q45, Q46, Q47, Q48, Q49, Q5, Q50, Q51, Q52, Q53, Q54, Q55, Q56, Q57, Q58, Q59, Q6, Q60, Q61, Q62, Q63, Q64, Q65, Q66, Q67, Q68, Q69, Q7, Q70, Q71, Q72, Q73, Q74, Q75, Q76, Q77, Q78, Q79, Q8, Q80, Q81, Q82, Q83, Q84, Q85, Q86, Q87, Q88, Q89, Q9, Q90, Q91, Q92, Q93, Q94, Q95, Q96, Q97, Q98, Q99: 2N7002, ellajameson-core:SOT23
- added R100, R101, R102, R103, R104, R105, R106, R107, R108, R109, R110, R111, R112, R113, R114, R115, R116, R117, R118, R119, R120, R121, R122, R123, R124, R125, R126, R127, R128, R129, R130, R131, R132, R25, R26, R27, R28, R29, R30, R31, R32, R33, R34, R35, R36, R37, R38, R39, R40, R41, R42, R43, R44, R45, R46, R47, R48, R49, R50, R51, R52, R53, R54, R55, R56, R57, R58, R59, R60, R61, R62, R63, R64, R65, R66, R67, R68, R69, R70, R71, R72, R73, R74, R79, R80, R83, R84, R87, R88, R91, R92, R95, R96, R97, R98, R99: 10k, ellajameson-core:R0603
- added R2, R3, R4, R5, R6, R7, R8, R9: 330, ellajameson-core:R0603
- added U$1, U$104, U$108, U$112, U$116, U$120, U$124, U$14, U$168, U$172, U$176, U$18, U$180, U$184, U$188, U$192, U$196, U$204, U$206, U$21, U$210, U$214, U$218, U$222, U$226, U$230, U$234, U$238, U$242, U$246, U$25, U$250, U$254, U$258, U$262, U$266, U$270, U$278, U$286, U$29, U$290, U$294, U$298, U$302, U$306, U$310, U$314, U$318, U$322, U$326, U$330, U$34, U$340, U$344, U$38, U$42, U$46, U$49, U$53, U$57, U$61, U$74, U$78, U$82, U$86, U$90, U$94: PROTOPADTHT, ellajameson-core:PROTOPAD-THT
- added U$10, U$105, U$106, U$109, U$110, U$113, U$114, U$117, U$118, U$12, U$121, U$122, U$125, U$126, U$134, U$136, U$15, U$16, U$169, U$170, U$173, U$174, U$177, U$178, U$181, U$182, U$185, U$186, U$189, U$19, U$190, U$193, U$194, U$197, U$198, U$2, U$20, U$201, U$205, U$207, U$208, U$211, U$212, U$215, U$216, U$219, U$22, U$220, U$223, U$224, U$227, U$228, U$23, U$231, U$232, U$235, U$236, U$239, U$240, U$243, U$244, U$247, U$248, U$251, U$252, U$255, U$256, U$259, U$26, U$260, U$263, U$264, U$267, U$268, U$27, U$271, U$272, U$274, U$275, U$279, U$280, U$283, U$287, U$288, U$291, U$292, U$295, U$296, U$299, U$3, U$30, U$300, U$303, U$304, U$307, U$308, U$31, U$311, U$312, U$315, U$316, U$319, U$320, U$323, U$324, U$327, U$328, U$331, U$332, U$341, U$342, U$345, U$346, U$35, U$36, U$39, U$40, U$43, U$44, U$47, U$48, U$5, U$50, U$51, U$54, U$55, U$58, U$59, U$62, U$63, U$65, U$67, U$69, U$7, U$71, U$75, U$76, U$79, U$80, U$83, U$84, U$87, U$88, U$91, U$92, U$95, U$96, U$98: (no value), ellajameson-core:PROTOPAD-BETWEEN
- added U$107, U$11, U$111, U$115, U$119, U$123, U$127, U$13, U$135, U$137, U$17, U$171, U$175, U$179, U$183, U$187, U$191, U$195, U$199, U$203, U$209, U$213, U$217, U$221, U$225, U$229, U$233, U$237, U$24, U$241, U$245, U$249, U$253, U$257, U$261, U$265, U$269, U$273, U$276, U$277, U$28, U$281, U$285, U$289, U$293, U$297, U$301, U$305, U$309, U$313, U$317, U$32, U$321, U$325, U$329, U$33, U$333, U$343, U$347, U$37, U$4, U$41, U$45, U$52, U$56, U$6, U$60, U$64, U$66, U$68, U$70, U$72, U$73, U$77, U$8, U$81, U$85, U$89, U$9, U$93, U$97, U$99: (no value), ellajameson-core:PROTOPAD-CENTER
- B1, B2, B3, B4, B5, B6, VCC1, VCC2, VCC3, VIN+1, VIN-1, VSS1, VSS2, VSS3: device ellajameson-core:PROTOPAD-THT -> ellajameson-core:PROTOPAD-THT-PAD
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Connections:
- new net N$10: D3.A, R3.1
- new net N$100: JP4.2, R27.1
- new net N$101: JN4.2, JS4.2, Q27.2, SOURCEA4.P1, SOURCEB4.P1
- new net N$102: DRAINA4.P1, DRAINB4.P1, JD3.1, JD4.2, JP4.1, JS51.1, Q27.3
- new net N$103: GATEA4.P1, GATEB4.P1, Q27.1
- new net N$104: JP5.2, R28.1
- new net N$105: JN5.2, JS5.2, Q28.2, SOURCEA5.P1, SOURCEB5.P1
- new net N$106: DRAINA5.P1, DRAINB5.P1, JD4.1, JD5.2, JP5.1, JS52.1, Q28.3
- new net N$107: GATEA5.P1, GATEB5.P1, Q28.1
- new net N$108: JP21.2, R29.1
- new net N$109: JN21.2, JS21.2, Q29.2, SOURCEA21.P1, SOURCEB21.P1
- new net N$11: LED3.P1, Q3.1
- new net N$110: DRAINA21.P1, DRAINB21.P1, JD21.2, JD5.1, JP21.1, JS53.1, Q29.3
- new net N$111: GATEA21.P1, GATEB21.P1, Q29.1
- new net N$112: JP22.2, R30.1
- new net N$113: JN22.2, JS22.2, Q30.2, SOURCEA22.P1, SOURCEB22.P1
- new net N$114: DRAINA22.P1, DRAINB22.P1, JD21.1, JD22.2, JP22.1, JS54.1, Q30.3
- new net N$115: GATEA22.P1, GATEB22.P1, Q30.1
- new net N$116: JP23.2, R31.1
- new net N$117: JN23.2, JS23.2, Q31.2, SOURCEA23.P1, SOURCEB23.P1
- new net N$118: DRAINA23.P1, DRAINB23.P1, JD22.1, JD23.2, JP23.1, JS55.1, Q31.3
- new net N$119: GATEA23.P1, GATEB23.P1, Q31.1
- new net N$12: D3.C, Q3.3
- new net N$120: JP24.2, R32.1
- new net N$121: JN24.2, JS24.2, Q32.2, SOURCEA24.P1, SOURCEB24.P1
- new net N$122: DRAINA24.P1, DRAINB24.P1, JD23.1, JD24.2, JP24.1, JS56.1, Q32.3
- new net N$123: GATEA24.P1, GATEB24.P1, Q32.1
- new net N$124: JP25.2, R33.1
- new net N$125: JN25.2, JS25.2, Q33.2, SOURCEA25.P1, SOURCEB25.P1
- new net N$126: DRAINA25.P1, DRAINB25.P1, JD24.1, JD25.2, JP25.1, JS57.1, Q33.3
- new net N$127: GATEA25.P1, GATEB25.P1, Q33.1
- new net N$128: JP26.2, R34.1
- new net N$129: JN26.2, JS26.2, Q34.2, SOURCEA26.P1, SOURCEB26.P1
- new net N$13: D4.A, R4.1
- new net N$130: DRAINA26.P1, DRAINB26.P1, JD25.1, JD26.2, JP26.1, JS58.1, Q34.3
- new net N$131: GATEA26.P1, GATEB26.P1, Q34.1
- new net N$132: JP27.2, R35.1
- new net N$133: JN27.2, JS27.2, Q35.2, SOURCEA27.P1, SOURCEB27.P1
- new net N$134: DRAINA27.P1, DRAINB27.P1, JD26.1, JD27.2, JP27.1, JS59.1, Q35.3
- new net N$135: GATEA27.P1, GATEB27.P1, Q35.1
- new net N$136: JP28.2, R36.1
- new net N$137: JN28.2, JS28.2, Q36.2, SOURCEA28.P1, SOURCEB28.P1
- new net N$138: DRAINA28.P1, DRAINB28.P1, JD27.1, JD28.2, JP28.1, JS60.1, Q36.3
- new net N$139: GATEA28.P1, GATEB28.P1, Q36.1
- new net N$14: LED4.P1, Q4.1
- new net N$140: JP29.2, R37.1
- new net N$141: JN29.2, JS29.2, Q37.2, SOURCEA29.P1, SOURCEB29.P1
- new net N$142: DRAINA29.P1, DRAINB29.P1, JD28.1, JD29.2, JP29.1, JS61.1, Q37.3
- new net N$143: GATEA29.P1, GATEB29.P1, Q37.1
- new net N$144: JP30.2, R38.1
- new net N$145: JN30.2, JS30.2, Q38.2, SOURCEA30.P1, SOURCEB30.P1
- new net N$146: DRAINA30.P1, DRAINB30.P1, JD29.1, JD30.2, JP30.1, JS62.1, Q38.3
- new net N$147: GATEA30.P1, GATEB30.P1, Q38.1
- new net N$148: JP31.2, R39.1
- new net N$149: JN31.2, JS31.2, Q39.2, SOURCEA31.P1, SOURCEB31.P1
- new net N$15: D4.C, Q4.3
- new net N$150: DRAINA31.P1, DRAINB31.P1, JD30.1, JD31.2, JP31.1, JS63.1, Q39.3
- new net N$151: GATEA31.P1, GATEB31.P1, Q39.1
- new net N$152: JP32.2, R40.1
- new net N$153: JN32.2, JS32.2, Q40.2, SOURCEA32.P1, SOURCEB32.P1
- new net N$154: DRAINA32.P1, DRAINB32.P1, JD31.1, JD32.2, JP32.1, JS64.1, Q40.3
- new net N$155: GATEA32.P1, GATEB32.P1, Q40.1
- new net N$156: JP33.2, R41.1
- new net N$157: JN33.2, JS33.2, Q41.2, SOURCEA33.P1, SOURCEB33.P1
- new net N$158: DRAINA33.P1, DRAINB33.P1, JD33.2, JP33.1, JS2.1, Q41.3
- new net N$159: GATEA33.P1, GATEB33.P1, Q41.1
- new net N$16: D5.A, R5.1
- new net N$160: JP34.2, R42.1
- new net N$161: JN34.2, JS34.2, Q42.2, SOURCEA34.P1, SOURCEB34.P1
- new net N$162: DRAINA34.P1, DRAINB34.P1, JD33.1, JD34.2, JP34.1, JS3.1, Q42.3
- new net N$163: GATEA34.P1, GATEB34.P1, Q42.1
- new net N$164: JP35.2, R43.1
- new net N$165: JN35.2, JS35.2, Q43.2, SOURCEA35.P1, SOURCEB35.P1
- new net N$166: DRAINA35.P1, DRAINB35.P1, JD34.1, JD35.2, JP35.1, JS4.1, Q43.3
- new net N$167: GATEA35.P1, GATEB35.P1, Q43.1
- new net N$168: JP36.2, R44.1
- new net N$169: JN36.2, JS36.2, Q44.2, SOURCEA36.P1, SOURCEB36.P1
- new net N$17: LED5.P1, Q5.1
- new net N$170: DRAINA36.P1, DRAINB36.P1, JD35.1, JD36.2, JP36.1, JS5.1, Q44.3
- new net N$171: GATEA36.P1, GATEB36.P1, Q44.1
- new net N$172: JP37.2, R45.1
- new net N$173: JN37.2, JS37.2, Q45.2, SOURCEA37.P1, SOURCEB37.P1
- new net N$174: DRAINA37.P1, DRAINB37.P1, JD36.1, JD37.2, JP37.1, JS21.1, Q45.3
- new net N$175: GATEA37.P1, GATEB37.P1, Q45.1
- new net N$176: JP38.2, R46.1
- new net N$177: JN38.2, JS38.2, Q46.2, SOURCEA38.P1, SOURCEB38.P1
- new net N$178: DRAINA38.P1, DRAINB38.P1, JD37.1, JD38.2, JP38.1, JS22.1, Q46.3
- new net N$179: GATEA38.P1, GATEB38.P1, Q46.1
- new net N$18: D5.C, Q5.3
- new net N$180: JP39.2, R47.1
- new net N$181: JN39.2, JS39.2, Q47.2, SOURCEA39.P1, SOURCEB39.P1
- new net N$182: DRAINA39.P1, DRAINB39.P1, JD38.1, JD39.2, JP39.1, JS23.1, Q47.3
- new net N$183: GATEA39.P1, GATEB39.P1, Q47.1
- new net N$184: JP40.2, R48.1
- new net N$185: JN40.2, JS40.2, Q48.2, SOURCEA40.P1, SOURCEB40.P1
- new net N$186: DRAINA40.P1, DRAINB40.P1, JD39.1, JD40.2, JP40.1, JS24.1, Q48.3
- new net N$187: GATEA40.P1, GATEB40.P1, Q48.1
- new net N$188: JP41.2, R49.1
- new net N$189: JN41.2, JS41.2, Q49.2, SOURCEA41.P1, SOURCEB41.P1
- new net N$19: D6.A, R6.1
- new net N$190: DRAINA41.P1, DRAINB41.P1, JD40.1, JD41.2, JP41.1, JS25.1, Q49.3
- new net N$191: GATEA41.P1, GATEB41.P1, Q49.1
- new net N$192: JP42.2, R50.1
- new net N$193: JN42.2, JS42.2, Q50.2, SOURCEA42.P1, SOURCEB42.P1
- new net N$194: DRAINA42.P1, DRAINB42.P1, JD41.1, JD42.2, JP42.1, JS26.1, Q50.3
- new net N$195: GATEA42.P1, GATEB42.P1, Q50.1
- new net N$196: JP43.2, R51.1
- new net N$197: JN43.2, JS43.2, Q51.2, SOURCEA43.P1, SOURCEB43.P1
- new net N$198: DRAINA43.P1, DRAINB43.P1, JD42.1, JD43.2, JP43.1, JS27.1, Q51.3
- new net N$199: GATEA43.P1, GATEB43.P1, Q51.1
- new net N$20: LED6.P1, Q6.1
- new net N$200: JP44.2, R52.1
- new net N$201: JN44.2, JS44.2, Q52.2, SOURCEA44.P1, SOURCEB44.P1
- new net N$202: DRAINA44.P1, DRAINB44.P1, JD43.1, JD44.2, JP44.1, JS28.1, Q52.3
- new net N$203: GATEA44.P1, GATEB44.P1, Q52.1
- new net N$204: JP45.2, R53.1
- new net N$205: JN45.2, JS45.2, Q53.2, SOURCEA45.P1, SOURCEB45.P1
- new net N$206: DRAINA45.P1, DRAINB45.P1, JD44.1, JD45.2, JP45.1, JS29.1, Q53.3
- new net N$207: GATEA45.P1, GATEB45.P1, Q53.1
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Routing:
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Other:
- board size 77.5 x 99.1 mm -> 83.8 x 99.1 mm
- board text added: "A#"
- board text added: "A1"
- board text added: "B#"
- board text added: "B1"
- board text added: "C#"
- board text added: "C1"
- board text added: "D"
- board text added: "D#"
- board text added: "D1"
- board text added: "E#"
- board text added: "E1"
- board text added: "F#"
- board text added: "F1"
- board text added: "G"
- board text added: "G#"
- board text added: "G1"
- board text added: "H#"
- board text added: "H1"
- board text added: "I#"
- board text added: "I1"
- board text added: "J#"
- board text added: "J1"
- board text added: "K#"
- board text added: "K1"
- board text added: "L#"
- board text added: "L1"
- board text added: "L2"
- board text added: "L3"
- board text added: "L4"
- board text added: "L5"
- board text added: "L6"
- board text added: "L7"
- board text added: "L8"
- board text added: "M#"
- board text added: "M1"
- board text added: "N#"
- board text added: "N1"
- board text added: "O#"
- board text added: "O1"
- board text added: "P#"
- board text added: "P1"
- board text added: "S"
